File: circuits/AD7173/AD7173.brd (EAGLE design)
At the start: 21 x 31.2 mm, 37 parts, among them IC1 AD7173, IC2 ADP1720, IC3 ADP1720ARMZ-5, IC4 ADR445BR, Q1 FA-20H

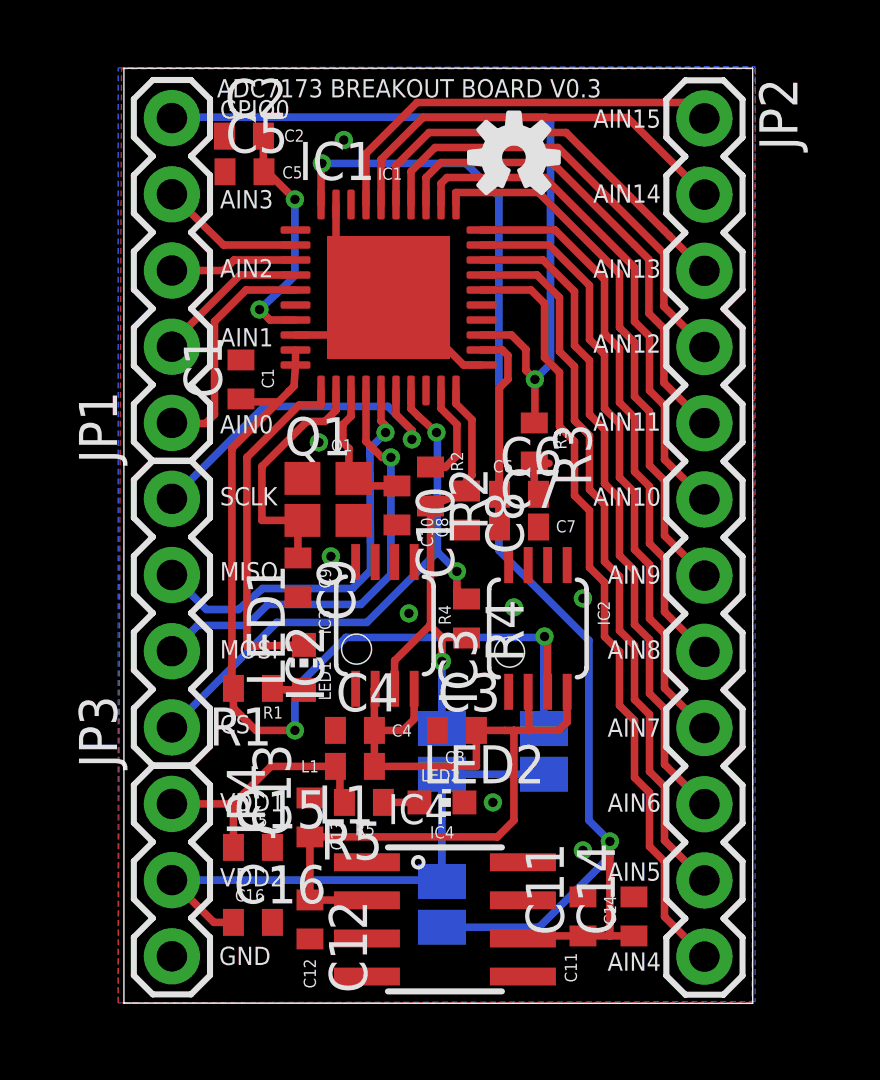
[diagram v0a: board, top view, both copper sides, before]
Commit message: small margin updates
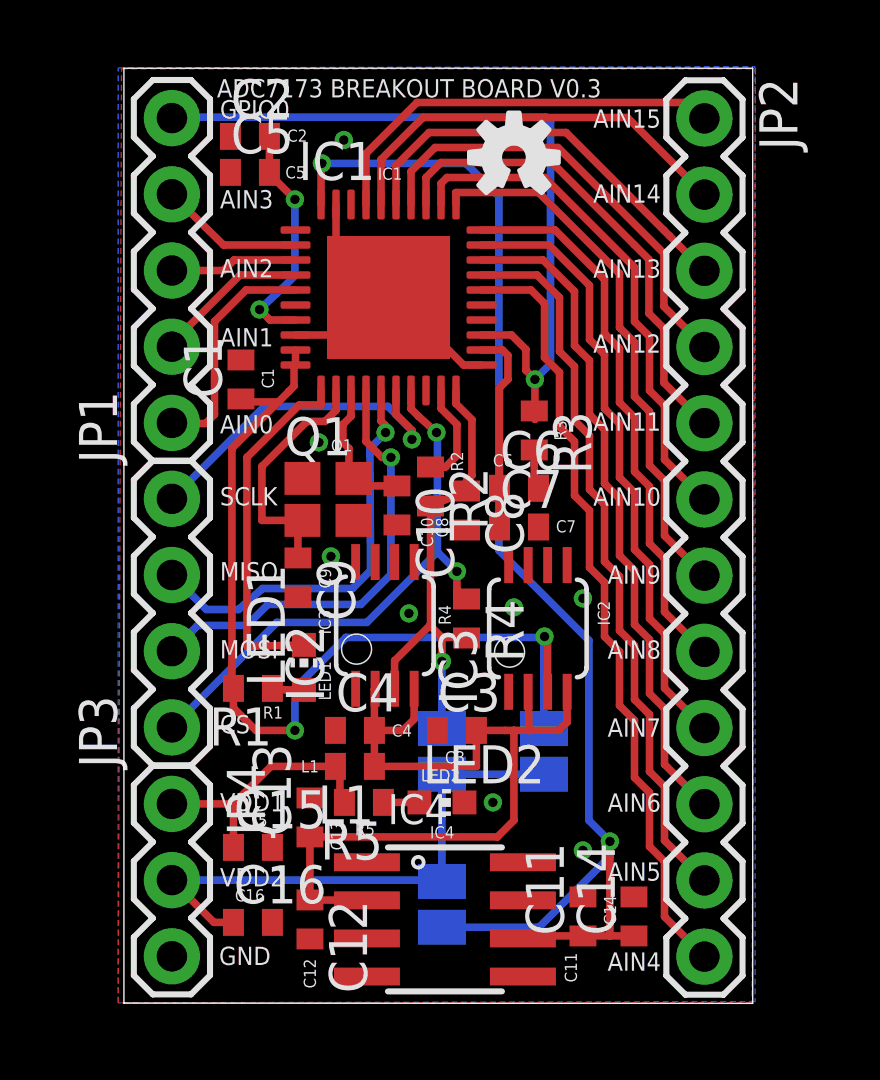
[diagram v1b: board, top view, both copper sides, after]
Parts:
- moved R3 0.40 mm to (13.9, 19.1)
- moved C2 0.20 mm to (4.40, 28.9)
- moved C6 0.20 mm to (13.4, 17.2)
- moved C5 0.18 mm to (4.40, 27.7)
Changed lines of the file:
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@@
 <wire x1="0.2" y1="31.174" x2="0.2" y2="0.01" width="0" layer="20"/>
 <text x="5.2" y="20.5" size="0.4064" layer="121" font="vector" ratio="10" rot="R90">C1</text>
-<text x="6.211803125" y="29.1289875" size="0.4064" layer="121" font="vector" ratio="10" rot="R180">C2</text>
+<text x="6.311803125" y="29.1289875" size="0.4064" layer="121" font="vector" ratio="10" rot="R180">C2</text>
 <text x="10.9" y="8" size="0.4064" layer="121" font="vector" ratio="10">C3</text>
 <text x="9.8" y="9.3" size="0.4064" layer="121" font="vector" ratio="10" rot="R180">C4</text>
@@
 <text x="5.5" y="9.9" size="0.4064" layer="121" font="vector" ratio="10" rot="R180">R1</text>
 <text x="11.1" y="18.4" size="0.4064" layer="121" font="vector" ratio="10" rot="R270">R2</text>
-<text x="14.5481875" y="19.131803125" size="0.4064" layer="121" font="vector" ratio="10" rot="R270">R3</text>
+<text x="14.5481875" y="19.431803125" size="0.4064" layer="121" font="vector" ratio="10" rot="R270">R3</text>
 <text x="3.4" y="26.5" size="0.6096" layer="121" font="vector" ratio="10">AIN3</text>
 <text x="3.4" y="24.2" size="0.6096" layer="121" font="vector" ratio="10">AIN2</text>
@@
 <text x="18.1" y="27.3" size="0.6096" layer="121" font="vector" ratio="10" rot="R180">AIN14</text>
 <text x="18.1" y="29.8" size="0.6096" layer="121" font="vector" ratio="10" rot="R180">AIN15</text>
-<text x="12.5" y="17.7" size="0.4064" layer="121" font="vector" ratio="10">C6</text>
+<text x="12.5" y="17.9" size="0.4064" layer="121" font="vector" ratio="10">C6</text>
 <text x="14.6" y="15.7" size="0.4064" layer="121" font="vector" ratio="10">C7</text>
 <text x="10.6" y="16.2" size="0.4064" layer="121" font="vector" ratio="10" rot="R270">C8</text>
@@
 <text x="7.1" y="12.3" size="0.4064" layer="121" font="vector" ratio="10" rot="R90">IC3</text>
 <text x="16.4" y="12.6" size="0.4064" layer="121" font="vector" ratio="10" rot="R90">IC2</text>
-<text x="5.48" y="27.5" size="0.4064" layer="121" font="vector" ratio="10">C5</text>
+<text x="5.58" y="27.5" size="0.4064" layer="121" font="vector" ratio="10">C5</text>
 <text x="3.37" y="1.28" size="0.6096" layer="121" font="vector" ratio="10">GND</text>
 <text x="3.3" y="30.2" size="0.6096" layer="121" font="vector" ratio="10">ADC7173 BREAKOUT BOARD V0.3</text>
@@
 <element name="C1" library="rcl" package="C0402" value="0.1uF" x="4.1" y="20.8" rot="R90"/>
 <element name="R2" library="rcl" package="R0402" value="10k" x="10.42" y="17.23" rot="R270"/>
-<element name="R3" library="rcl" package="R0402" value="10k" x="13.88" y="18.7" rot="R270"/>
-<element name="C2" library="rcl" package="C0402" value="0.1uF" x="4.2" y="28.91"/>
+<element name="R3" library="rcl" package="R0402" value="10k" x="13.88" y="19.1" rot="R270"/>
+<element name="C2" library="rcl" package="C0402" value="0.1uF" x="4.4" y="28.9"/>
 <element name="C3" library="rcl" package="C0402" value="4.7uF" x="11.3" y="9.1"/>
-<element name="C5" library="rcl" package="C0402" value="1uF" x="4.22" y="27.72"/>
-<element name="C6" library="rcl" package="C0402" value="0.1uF" x="13.37" y="16.97"/>
+<element name="C5" library="rcl" package="C0402" value="1uF" x="4.4" y="27.7"/>
+<element name="C6" library="rcl" package="C0402" value="0.1uF" x="13.37" y="17.17"/>
 <element name="C7" library="rcl" package="C0402" value="1uF" x="13.37" y="15.88"/>
 <element name="C8" library="rcl" package="C0402" value="0.1uF" x="11.62" y="16.43" rot="R270"/>
@@
 <via x="12.5" y="6.7" extent="1-16" drill="0.31"/>
 <via x="15.5" y="13.5" extent="1-16" drill="0.31"/>
-<wire x1="14.37" y1="18" x2="13.88" y2="18.05" width="0.254" layer="1"/>
 <contactref element="C16" pad="2"/>
 <via x="15.5" y="5.1" extent="1-16" drill="0.31"/>
-<wire x1="14.02" y1="16.97" x2="13.88" y2="17.11" width="0.254" layer="1"/>
-<wire x1="13.88" y1="17.11" x2="13.88" y2="18.05" width="0.254" layer="1"/>
+<wire x1="14.02" y1="17.17" x2="13.88" y2="17.11" width="0.254" layer="1"/>
+<wire x1="13.88" y1="17.11" x2="13.88" y2="18.45" width="0.254" layer="1"/>
 <contactref element="JP4" pad="3"/>
 <via x="9.7" y="13" extent="1-16" drill="0.31"/>
@@
 <contactref element="R1" pad="2"/>
 <wire x1="5.92" y1="21.78" x2="5.92" y2="21.28" width="0.254" layer="1"/>
-<wire x1="5.92" y1="21.28" x2="5.87" y2="20.58" width="0.254" layer="1"/>
 <wire x1="5.87" y1="20.58" x2="5.7" y2="20.4" width="0.254" layer="1"/>
 <wire x1="5.7" y1="20.4" x2="5.35" y2="20.05" width="0.254" layer="1"/>
@@
 <wire x1="14.22" y1="12.23" x2="14.324" y2="12.126" width="0.254" layer="1"/>
 <wire x1="14.324" y1="12.126" x2="14.324" y2="10.387" width="0.254" layer="1"/>
+<wire x1="5.92" y1="21.28" x2="5.87" y2="21.28" width="0.254" layer="1"/>
+<wire x1="5.87" y1="21.28" x2="5.87" y2="20.58" width="0.254" layer="1"/>
 </signal>
 <signal name="N$3">
@@
 <wire x1="13.9" y1="20.8" x2="14.42" y2="21.32" width="0.254" layer="16"/>
 <wire x1="14.42" y1="21.32" x2="14.42" y2="29.38" width="0.254" layer="16"/>
-<wire x1="13.88" y1="19.35" x2="13.9" y2="19.47" width="0.254" layer="1"/>
+<wire x1="13.88" y1="19.75" x2="13.9" y2="19.47" width="0.254" layer="1"/>
 <wire x1="13.9" y1="19.47" x2="13.9" y2="20.8" width="0.254" layer="1"/>
 </signal>
@@
 <via x="5.9" y="26.8" extent="1-16" drill="0.31"/>
 <wire x1="5.9" y1="26.8" x2="4.98" y2="27.72" width="0.254" layer="1"/>
-<wire x1="4.98" y1="27.72" x2="4.87" y2="27.72" width="0.254" layer="1"/>
-<wire x1="4.87" y1="27.72" x2="4.85" y2="27.74" width="0.254" layer="1"/>
-<wire x1="4.85" y1="27.74" x2="4.85" y2="28.91" width="0.254" layer="1"/>
+<wire x1="4.98" y1="27.72" x2="5.05" y2="27.7" width="0.254" layer="1"/>
+<wire x1="5.05" y1="27.7" x2="5.05" y2="28.9" width="0.254" layer="1"/>
 </signal>
 <signal name="N$38">
@@
 <contactref element="IC1" pad="22"/>
 <wire x1="13" y1="20.8" x2="12.72" y2="20.52" width="0.254" layer="1"/>
-<wire x1="12.72" y1="20.52" x2="12.72" y2="16.97" width="0.254" layer="1"/>
-<wire x1="12.72" y1="16.97" x2="12.72" y2="15.88" width="0.254" layer="1"/>
+<wire x1="12.72" y1="20.52" x2="12.72" y2="17.17" width="0.254" layer="1"/>
+<wire x1="12.72" y1="17.17" x2="12.72" y2="15.88" width="0.254" layer="1"/>
 <wire x1="12.12" y1="21.78" x2="12.82" y2="21.78" width="0.254" layer="1"/>
 <wire x1="12.82" y1="21.78" x2="13" y2="21.6" width="0.254" layer="1"/>
